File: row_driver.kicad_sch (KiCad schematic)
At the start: 22 parts, among them SW3 SW_PUSH_SMALL_H, SW4 SW_PUSH_SMALL_H, SW5 SW_PUSH_SMALL_H, SW6 SW_PUSH_SMALL_H, SW7 SW_PUSH_SMALL_H, SW8 SW_PUSH_SMALL_H, U11 74HC595, U13 74HC595, U15 74HC595, U23 CM1293A-04SO, U24 CM1293A-04SO

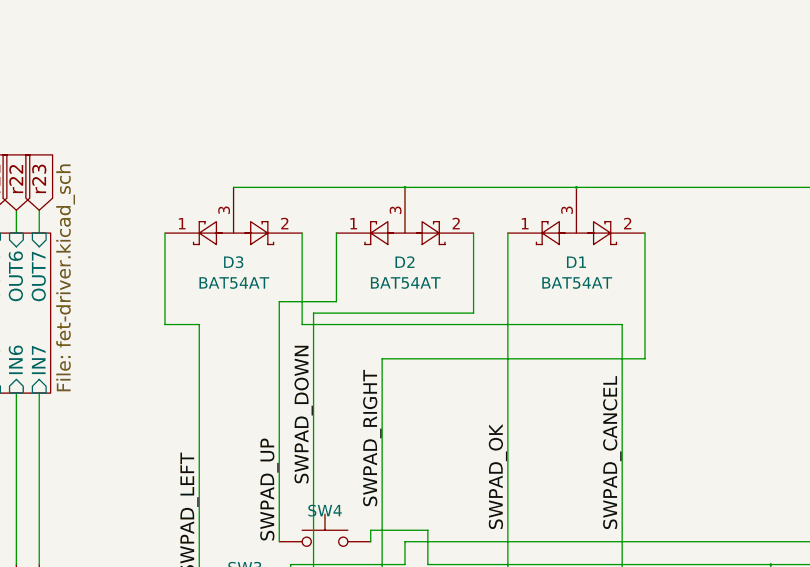
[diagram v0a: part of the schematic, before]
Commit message: Revert "Modified BAT54A -> BAT54AT"
This reverts commit bff826c2a0df659e4b46f46fdcd99af7f60e1fdb.
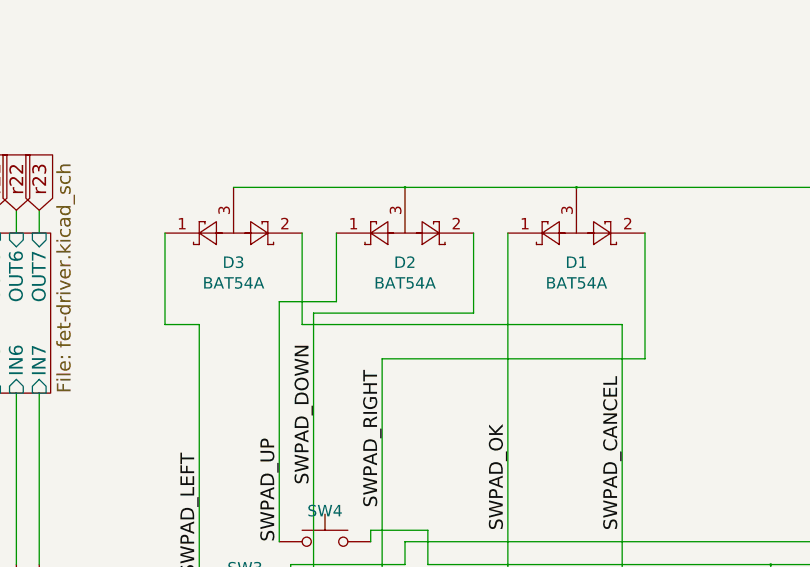
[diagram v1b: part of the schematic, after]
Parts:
- D1, D2, D3: value BAT54AT -> BAT54A; footprint components:SOT-523-handsoldering -> Package_TO_SOT_SMD:SOT-23_Handsoldering
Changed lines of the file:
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@@
     (in_bom yes) (on_board yes)
     (property "Reference" "D3" (id 0) (at 146.05 43.923 0))
-    (property "Value" "BAT54AT" (id 1) (at 146.05 46.2217 0))
-    (property "Footprint" "components:SOT-523-handsoldering" (id 2) (at 147.955 43.815 0)
+    (property "Value" "BAT54A" (id 1) (at 146.05 46.2217 0))
+    (property "Footprint" "Package_TO_SOT_SMD:SOT-23_Handsoldering" (id 2) (at 147.955 43.815 0)
       (effects (font (size 1.27 1.27)) (justify left) hide)
     )
@@
     (in_bom yes) (on_board yes)
     (property "Reference" "D2" (id 0) (at 165.1 43.923 0))
-    (property "Value" "BAT54AT" (id 1) (at 165.1 46.2217 0))
-    (property "Footprint" "components:SOT-523-handsoldering" (id 2) (at 167.005 43.815 0)
+    (property "Value" "BAT54A" (id 1) (at 165.1 46.2217 0))
+    (property "Footprint" "Package_TO_SOT_SMD:SOT-23_Handsoldering" (id 2) (at 167.005 43.815 0)
       (effects (font (size 1.27 1.27)) (justify left) hide)
     )
@@
     (in_bom yes) (on_board yes)
     (property "Reference" "D1" (id 0) (at 184.15 43.923 0))
-    (property "Value" "BAT54AT" (id 1) (at 184.15 46.2217 0))
-    (property "Footprint" "components:SOT-523-handsoldering" (id 2) (at 186.055 43.815 0)
+    (property "Value" "BAT54A" (id 1) (at 184.15 46.2217 0))
+    (property "Footprint" "Package_TO_SOT_SMD:SOT-23_Handsoldering" (id 2) (at 186.055 43.815 0)
       (effects (font (size 1.27 1.27)) (justify left) hide)
     )

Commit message: Modified BAT54A -> BAT54AT
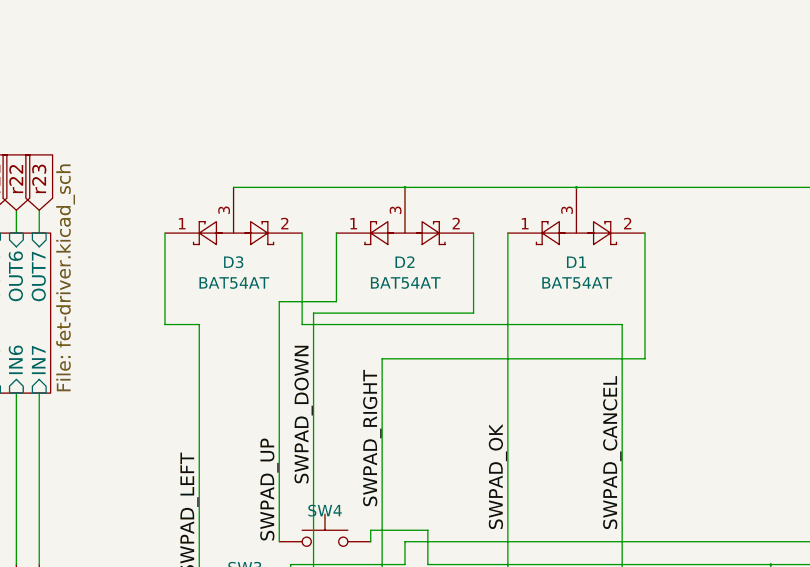
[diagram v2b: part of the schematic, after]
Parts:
- D1, D2, D3: value BAT54A -> BAT54AT; footprint Package_TO_SOT_SMD:SOT-23_Handsoldering -> components:SOT-523-handsoldering
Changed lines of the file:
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@@
     (in_bom yes) (on_board yes)
     (property "Reference" "D3" (id 0) (at 146.05 43.923 0))
-    (property "Value" "BAT54A" (id 1) (at 146.05 46.2217 0))
-    (property "Footprint" "Package_TO_SOT_SMD:SOT-23_Handsoldering" (id 2) (at 147.955 43.815 0)
+    (property "Value" "BAT54AT" (id 1) (at 146.05 46.2217 0))
+    (property "Footprint" "components:SOT-523-handsoldering" (id 2) (at 147.955 43.815 0)
       (effects (font (size 1.27 1.27)) (justify left) hide)
     )
@@
     (in_bom yes) (on_board yes)
     (property "Reference" "D2" (id 0) (at 165.1 43.923 0))
-    (property "Value" "BAT54A" (id 1) (at 165.1 46.2217 0))
-    (property "Footprint" "Package_TO_SOT_SMD:SOT-23_Handsoldering" (id 2) (at 167.005 43.815 0)
+    (property "Value" "BAT54AT" (id 1) (at 165.1 46.2217 0))
+    (property "Footprint" "components:SOT-523-handsoldering" (id 2) (at 167.005 43.815 0)
       (effects (font (size 1.27 1.27)) (justify left) hide)
     )
@@
     (in_bom yes) (on_board yes)
     (property "Reference" "D1" (id 0) (at 184.15 43.923 0))
-    (property "Value" "BAT54A" (id 1) (at 184.15 46.2217 0))
-    (property "Footprint" "Package_TO_SOT_SMD:SOT-23_Handsoldering" (id 2) (at 186.055 43.815 0)
+    (property "Value" "BAT54AT" (id 1) (at 184.15 46.2217 0))
+    (property "Footprint" "components:SOT-523-handsoldering" (id 2) (at 186.055 43.815 0)
       (effects (font (size 1.27 1.27)) (justify left) hide)
     )
